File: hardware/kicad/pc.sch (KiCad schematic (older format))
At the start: 16 parts

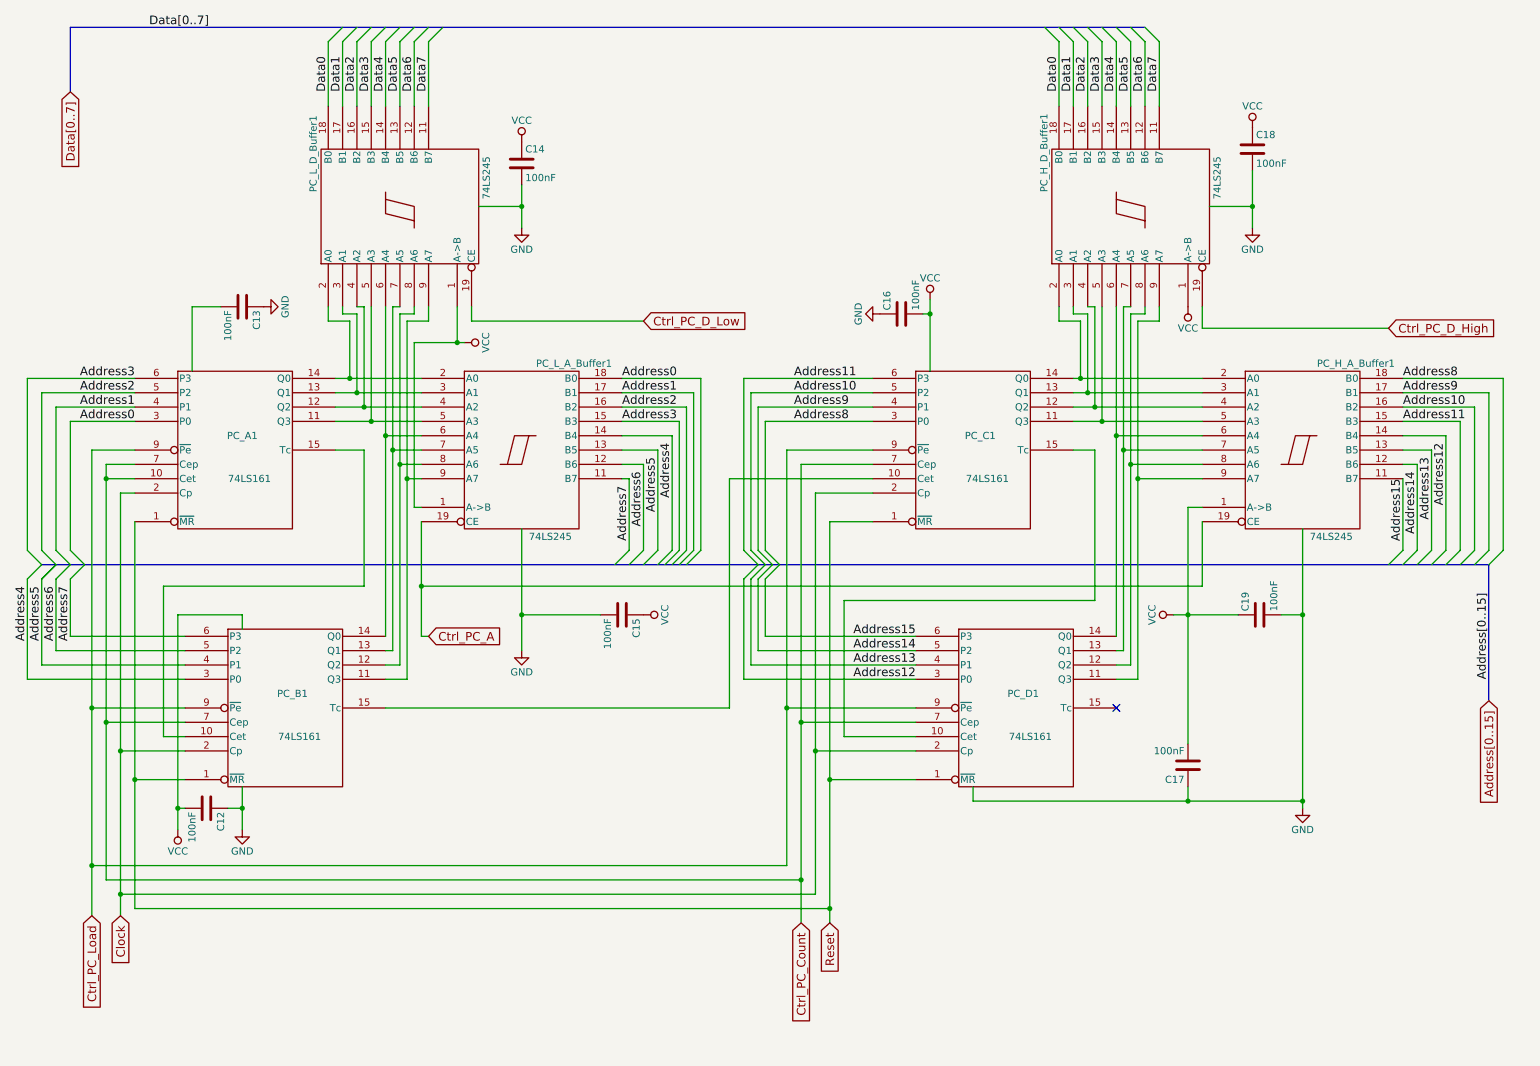
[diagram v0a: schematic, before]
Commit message: Just a backup.
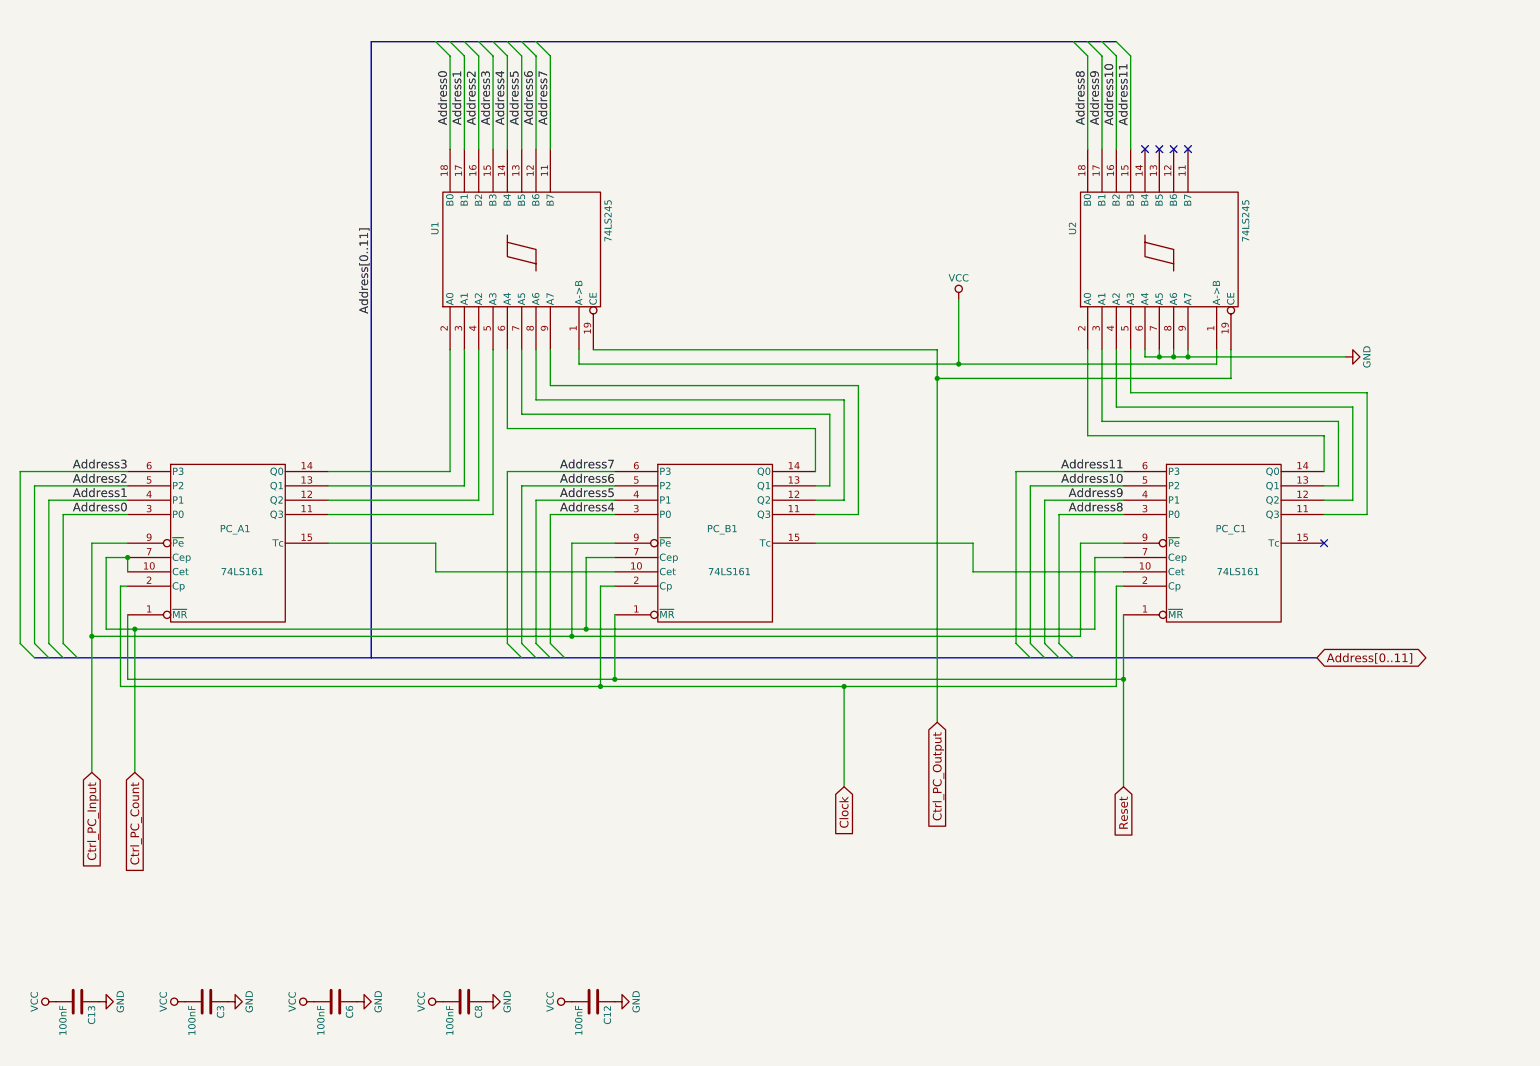
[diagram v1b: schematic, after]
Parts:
- removed C14, C15, C16, C17, C18, C19: 100nF, Capacitors_THT:C_Disc_D5.0mm_W2.5mm_P2.50mm, symbol C
- removed PC_D1: 74LS161, Housings_DIP:DIP-16_W7.62mm, symbol 74LS161
- removed PC_H_A_Buffer1, PC_H_D_Buffer1, PC_L_A_Buffer1, PC_L_D_Buffer1: 74LS245, Housings_DIP:DIP-20_W7.62mm, symbol 74LS245
- added C3, C6, C8: 100nF, Capacitors_ThroughHole:C_Disc_D3_P2.5, symbol C
- added U1, U2: 74LS245, Housings_DIP:DIP-20_W7.62mm, symbol 74LS245
- C12, C13: footprint Capacitors_THT:C_Disc_D5.0mm_W2.5mm_P2.50mm -> Capacitors_ThroughHole:C_Disc_D3_P2.5
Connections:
- net Address0: now also U1.18 (B0)
- net Address1: now also U1.17 (B1)
- net Address10: now also U2.16 (B2)
- net Address11: now also U2.15 (B3)
- net Address2: now also U1.16 (B2)
- net Address3: now also U1.15 (B3)
- net Address4: now also U1.14 (B4)
- net Address5: now also U1.13 (B5)
- net Address6: now also U1.12 (B6)
- net Address7: now also U1.11 (B7)
- net Address8: now also U2.18 (B0)
- net Address9: now also U2.17 (B1)
- net GND: now also C3.1, C6.1, C8.1, U1.10 (GND), U2.10 (GND), U2.6 (A4), U2.7 (A5), U2.8 (A6), U2.9 (A7)
- net VCC: now also C3.2, C6.2, C8.2, U1.1 (A->B), U1.20 (VCC), U2.1 (A->B), U2.20 (VCC)
- net at PC_A1.11 (Q3): now also U1.5 (A3)
- net at PC_A1.12 (Q2): now also U1.4 (A2)
- net at PC_A1.13 (Q1): now also U1.3 (A1)
- net at PC_A1.14 (Q0): now also U1.2 (A0)
- net at PC_B1.11 (Q3): now also U1.9 (A7)
- net at PC_B1.12 (Q2): now also U1.8 (A6)
- net at PC_B1.13 (Q1): now also U1.7 (A5)
- net at PC_B1.14 (Q0): now also U1.6 (A4)
- net at PC_C1.11 (Q3): now also U2.5 (A3)
- net at PC_C1.12 (Q2): now also U2.4 (A2)
- net at PC_C1.13 (Q1): now also U2.3 (A1)
- net at PC_C1.14 (Q0): now also U2.2 (A0)
- net Ctrl_PC_Load renamed Ctrl_PC_Input
- new net Ctrl_PC_Output: U1.19 (CE), U2.19 (CE)
- no-connect marks 1 -> 5
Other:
- moved on the sheet: C13, PC_A1

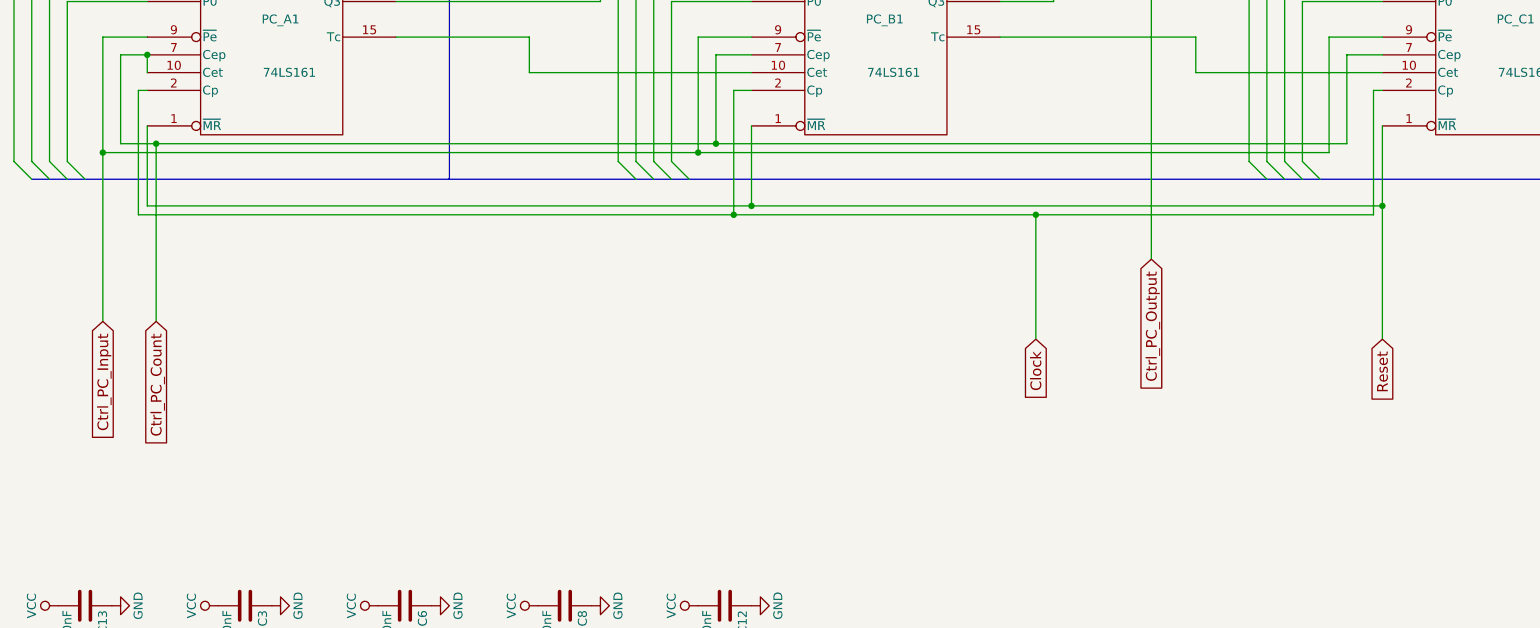
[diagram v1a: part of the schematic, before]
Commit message: Just a backup.
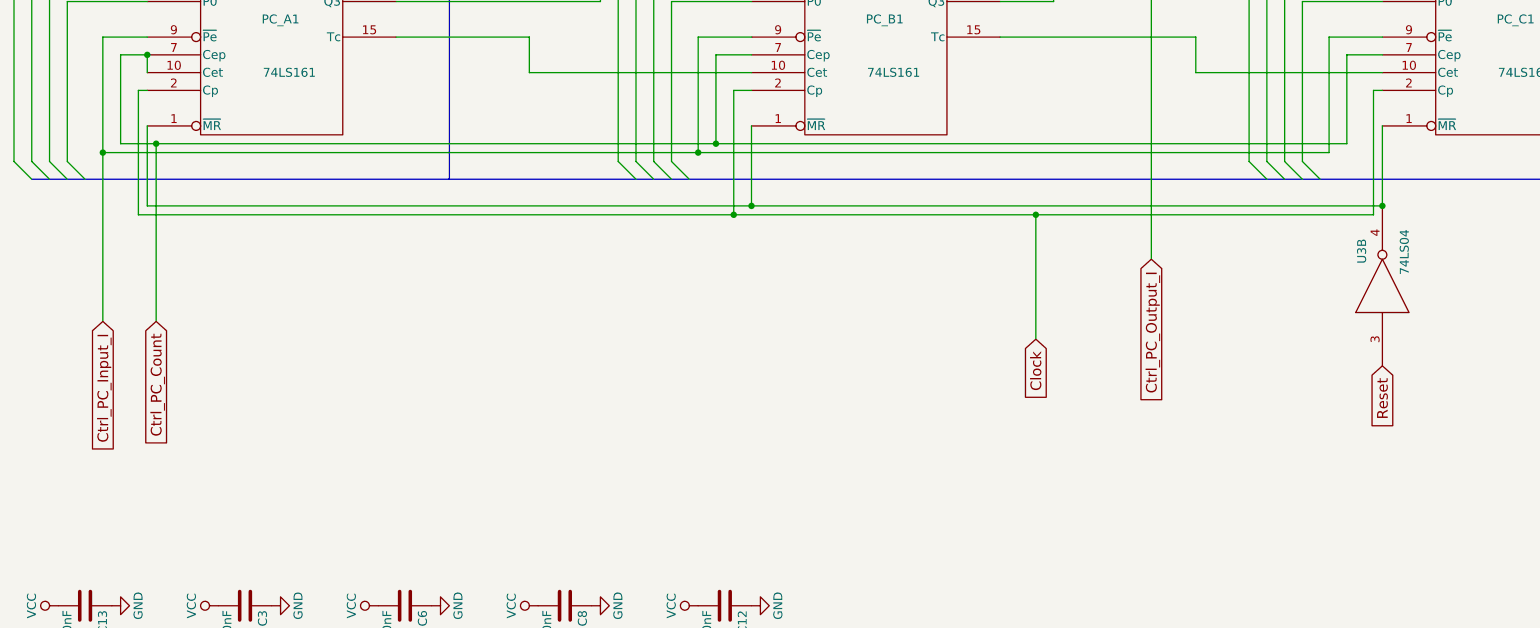
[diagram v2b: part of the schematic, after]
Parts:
- added U3: 74LS04, Housings_DIP:DIP-14_W7.62mm, symbol 74LS04
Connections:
- net GND: now also U3.7 (GND)
- net Reset: now also U3.3; no longer PC_A1.1 (~MR), PC_B1.1 (~MR), PC_C1.1 (~MR)
- net VCC: now also U3.14 (VCC)
- net Ctrl_PC_Input renamed Ctrl_PC_Input_I
- net Ctrl_PC_Output renamed Ctrl_PC_Output_I
- new net: PC_A1.1 (~MR), PC_B1.1 (~MR), PC_C1.1 (~MR), U3.4
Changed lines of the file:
@@
 Address[0..11]
 Text GLabel 1200 5800 3    60   Input ~ 0
-Ctrl_PC_Input
+Ctrl_PC_Input_I
 Text GLabel 1500 5800 3    60   Input ~ 0
 Ctrl_PC_Count
 Text GLabel 6450 5900 3    60   Input ~ 0
 Clock
-Text GLabel 8400 5900 3    60   Input ~ 0
+Text GLabel 8400 6050 3    60   Input ~ 0
 Reset
 Text Label 1450 4000 2    60   ~ 0
@@
 $EndComp
 $Comp
-L GND #PWR019
+L GND #PWR14
 U 1 1 5A1440E6
 P 1250 7400
-F 0 "#PWR019" H 1250 7150 50  0001 C CNN
+F 0 "#PWR14" H 1250 7150 50  0001 C CNN
 F 1 "GND" H 1250 7250 50  0000 C CNN
 F 2 "" H 1250 7400 50  0001 C CNN
@@
 Address11
 $Comp
-L VCC #PWR020
+L VCC #PWR13
 U 1 1 5BB5434D
 P 950 7400
-F 0 "#PWR020" H 950 7250 50  0001 C CNN
+F 0 "#PWR13" H 950 7250 50  0001 C CNN
 F 1 "VCC" H 950 7550 50  0000 C CNN
 F 2 "" H 950 7400 50  0000 C CNN
@@
 $EndComp
 $Comp
-L GND #PWR021
+L GND #PWR16
 U 1 1 5BB54403
 P 2150 7400
-F 0 "#PWR021" H 2150 7150 50  0001 C CNN
+F 0 "#PWR16" H 2150 7150 50  0001 C CNN
 F 1 "GND" H 2150 7250 50  0000 C CNN
 F 2 "" H 2150 7400 50  0001 C CNN
@@
 $EndComp
 $Comp
-L VCC #PWR022
+L VCC #PWR15
 U 1 1 5BB54409
 P 1850 7400
-F 0 "#PWR022" H 1850 7250 50  0001 C CNN
+F 0 "#PWR15" H 1850 7250 50  0001 C CNN
 F 1 "VCC" H 1850 7550 50  0000 C CNN
 F 2 "" H 1850 7400 50  0000 C CNN
@@
 $EndComp
 $Comp
-L GND #PWR023
+L GND #PWR18
 U 1 1 5BB54622
 P 3050 7400
-F 0 "#PWR023" H 3050 7150 50  0001 C CNN
+F 0 "#PWR18" H 3050 7150 50  0001 C CNN
 F 1 "GND" H 3050 7250 50  0000 C CNN
 F 2 "" H 3050 7400 50  0001 C CNN
@@
 $EndComp
 $Comp
-L VCC #PWR024
+L VCC #PWR17
 U 1 1 5BB54628
 P 2750 7400
-F 0 "#PWR024" H 2750 7250 50  0001 C CNN
+F 0 "#PWR17" H 2750 7250 50  0001 C CNN
 F 1 "VCC" H 2750 7550 50  0000 C CNN
 F 2 "" H 2750 7400 50  0000 C CNN
@@
 	10100 4000 9800 4000
 Text GLabel 7100 5450 3    60   Input ~ 0
-Ctrl_PC_Output
+Ctrl_PC_Output_I
 Wire Wire Line
 	4700 2850 7100 2850
@@
 	1450 5150 8400 5150
 Wire Wire Line
-	8400 4700 8400 5900
-Wire Wire Line
 	4850 4700 4850 5150
 Connection ~ 4850 5150
@@
 $EndComp
 $Comp
-L GND #PWR025
+L GND #PWR20
 U 1 1 5BB5C790
 P 3950 7400
-F 0 "#PWR025" H 3950 7150 50  0001 C CNN
+F 0 "#PWR20" H 3950 7150 50  0001 C CNN
 F 1 "GND" H 3950 7250 50  0000 C CNN
 F 2 "" H 3950 7400 50  0001 C CNN
@@
 $EndComp
 $Comp
-L VCC #PWR026
+L VCC #PWR19
 U 1 1 5BB5C796
 P 3650 7400
-F 0 "#PWR026" H 3650 7250 50  0001 C CNN
+F 0 "#PWR19" H 3650 7250 50  0001 C CNN
 F 1 "VCC" H 3650 7550 50  0000 C CNN
 F 2 "" H 3650 7400 50  0000 C CNN
@@
 $EndComp
 $Comp
-L GND #PWR027
+L GND #PWR22
 U 1 1 5BB5C7A2
 P 4850 7400
-F 0 "#PWR027" H 4850 7150 50  0001 C CNN
+F 0 "#PWR22" H 4850 7150 50  0001 C CNN
 F 1 "GND" H 4850 7250 50  0000 C CNN
 F 2 "" H 4850 7400 50  0001 C CNN
@@
 $EndComp
 $Comp
-L VCC #PWR028
+L VCC #PWR21
 U 1 1 5BB5C7A8
 P 4550 7400
-F 0 "#PWR028" H 4550 7250 50  0001 C CNN
+F 0 "#PWR21" H 4550 7250 50  0001 C CNN
 F 1 "VCC" H 4550 7550 50  0000 C CNN
 F 2 "" H 4550 7400 50  0000 C CNN
@@
 Address10
 $Comp
-L VCC #PWR029
+L VCC #PWR23
 U 1 1 5BB61853
 P 7250 2500
-F 0 "#PWR029" H 7250 2350 50  0001 C CNN
+F 0 "#PWR23" H 7250 2350 50  0001 C CNN
 F 1 "VCC" H 7250 2650 50  0000 C CNN
 F 2 "" H 7250 2500 50  0000 C CNN
@@
 Connection ~ 8850 2900
 $Comp
-L GND #PWR030
+L GND #PWR24
 U 1 1 5BB635A4
 P 9950 2900
-F 0 "#PWR030" H 9950 2650 50  0001 C CNN
+F 0 "#PWR24" H 9950 2650 50  0001 C CNN
 F 1 "GND" H 9950 2750 50  0000 C CNN
 F 2 "" H 9950 2900 50  0000 C CNN
@@
 Wire Wire Line
 	8550 2850 8550 2900
+Wire Wire Line
+	8400 5150 8400 4700
+$Comp
+L 74LS04 U3
+U 2 1 5BB827EB
+P 8400 5600
+F 0 "U3" H 8595 5715 50  0000 C CNN
+F 1 "74LS04" H 8590 5475 50  0000 C CNN
+F 2 "Housings_DIP:DIP-14_W7.62mm" H 8400 5600 50  0001 C CNN
+F 3 "" H 8400 5600 50  0000 C CNN
+	2    8400 5600
+	0    -1   -1   0
+$EndComp
 $EndSCHEMATC
